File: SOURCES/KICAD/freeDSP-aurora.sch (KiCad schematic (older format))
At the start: 76 parts, among them IC101 IC_ADAU1452, IC102 IC_25AA1024, IC103 IC_TLE2426ID, IC104 IC_ADM811TARTZ, IC105 IC_LM1117MP-5.0, IC106 IC_NCP1117LPST33, IC107 IC_LM1117MP-5.0, IC108 IC_LM1117MPX-ADJ, Q101 Q_STD2805, X101 MicroMatch14, X102 HDR_02x08, X103 HDR_01x03, X104 CON_MicroMatch-10G, X105 CON_MicroFit3_02x02, Y101 24M576

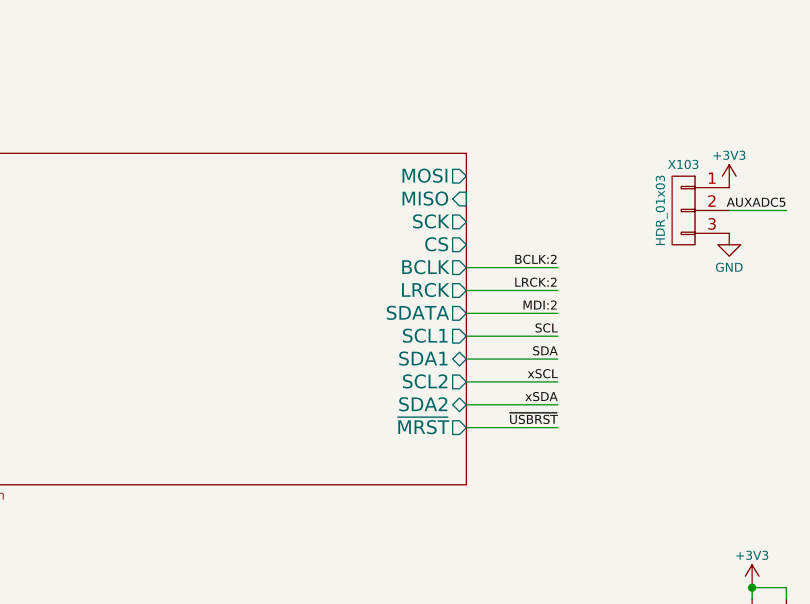
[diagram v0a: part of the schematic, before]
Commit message: Updated BOM
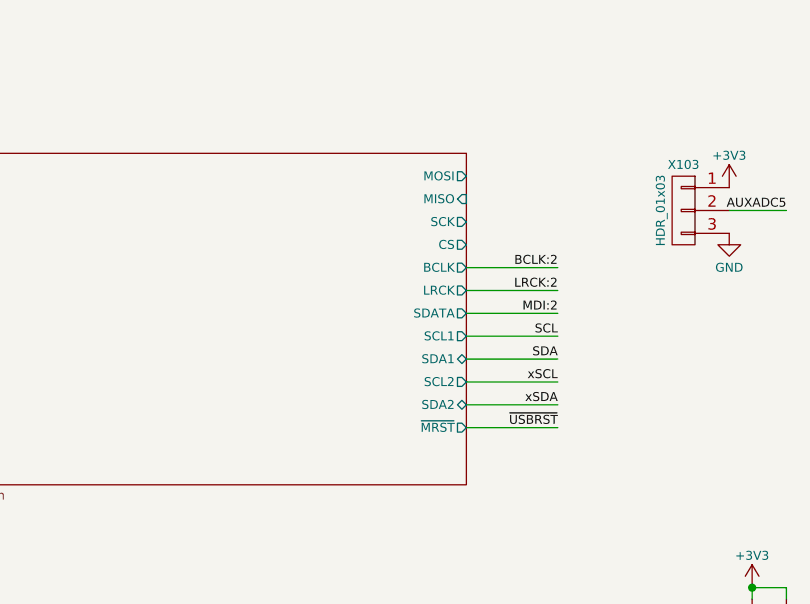
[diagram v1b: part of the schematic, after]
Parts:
- C101: Manufacturer (none) -> Murata Electronics North America; manf_num (none) -> GRM21BR61E106MA73L; pn (none) -> GRM21BR61E106MA73L
- C102, C105, C109, C110, C113, C118, C121, C124, C128, C129, C130, C131, C133, C134, C135, C136: Manufacturer (none) -> KEMET; pn (none) -> C0805C104K5RACTU
- C103: Manufacturer (none) -> Yageo; pn (none) -> CC0805KRX7R9BB562
- C104, C111, C112, C114, C117, C119, C120, C122, C123, C125, C127, C132, C137: Manufacturer (none) -> Murata Electronics North America; pn (none) -> GRM21BR61E106MA73L
- C106: Manufacturer (none) -> KEMET; pn (none) -> C0805C151J5GACTU
- C107, C108: Manufacturer (none) -> KEMET; pn (none) -> C0805C220J5GACTU
- C115, C116, C126: Manufacturer (none) -> Wurth Electronics Inc.; pn (none) -> 860010474012
- FER101, FER102: Manufacturer (none) -> Murata Electronics North America; pn (none) -> BLM21AG601SN1D
- IC101: Manufacturer (none) -> Analog Devices Inc.; pn (none) -> ADAU1452WBCPZ
- IC102: Manufacturer (none) -> Microchip Technology; pn (none) -> 25AA1024T-I/SM
- IC103: Manufacturer (none) -> Texas Instruments; pn (none) -> TLE2426IDR
- IC104: Manufacturer (none) -> Analog Devices Inc.; pn (none) -> ADM811TARTZ-REEL
- IC105, IC107: Manufacturer (none) -> Texas Instruments; pn (none) -> LM1117MP-5.0/NOPB
- IC106: Manufacturer (none) -> ON Semiconductor; pn (none) -> NCP1117LPST33T3G
- IC108: Manufacturer (none) -> Texas Instruments; pn (none) -> LM1117MPX-ADJ/NOPB
- JP101: Manufacturer (none) -> Wurth Electronics Inc.; pn (none) -> 61300211121
- Q101: Manufacturer (none) -> STMicroelectronics; pn (none) -> STD2805T4
- R101, R102, R104, R105: Manufacturer (none) -> Yageo; pn (none) -> TC164-JR-0733RL
- R103, R114: Manufacturer (none) -> Yageo; pn (none) -> RC0805FR-071KL
- R106: Manufacturer (none) -> Yageo; pn (none) -> RC0805FR-074K32L
- R107, R112, R113: Manufacturer (none) -> Yageo; pn (none) -> RC0805FR-0710KL
- R108: Manufacturer (none) -> Yageo; pn (none) -> RC0805FR-07100RL
- R109: Manufacturer (none) -> Yageo; pn (none) -> RC0805FR-0733RL
- R110, R111: Manufacturer (none) -> Yageo; pn (none) -> RC0805FR-072KL
- R115: Manufacturer (none) -> Yageo; pn (none) -> RC0805FR-07100KL
- R116: Manufacturer (none) -> Stackpole Electronics Inc.; pn (none) -> RNCP0805FTD150R
- R117: Manufacturer (none) -> Yageo; pn (none) -> RC0805FR-07931RL
- X101: Manufacturer (none) -> TE Connectivity AMP Connectors; pn (none) -> 1-215079-4
- X102: Manufacturer (none) -> Sullins Connector Solutions; pn (none) -> PRPC008DAAN-RC
- X103: Manufacturer (none) -> Sullins Connector Solutions; pn (none) -> PRPC003SAAN-RC
- X104: Manufacturer (none) -> TE Connectivity AMP Connectors; pn (none) -> 1-215079-0
- X105: Manufacturer (none) -> Molex, LLC; pn (none) -> 0430450428
- Y101: Manufacturer (none) -> EPSON; pn (none) -> FA-238 24.5760MB-K3
